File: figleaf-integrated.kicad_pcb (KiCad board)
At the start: 2 copper layers, 145 x 106 mm, 70 parts, among them J2 HRO_TYPE-C-31-M-14, J3 Battery, J9 TC2030_SWD, Q2 2N7002, SW1 PWR, SW2 RST, U1 SRV05-4, U10 MAX17048, U3 BQ24075, U8 nRF52840_moko_mk08

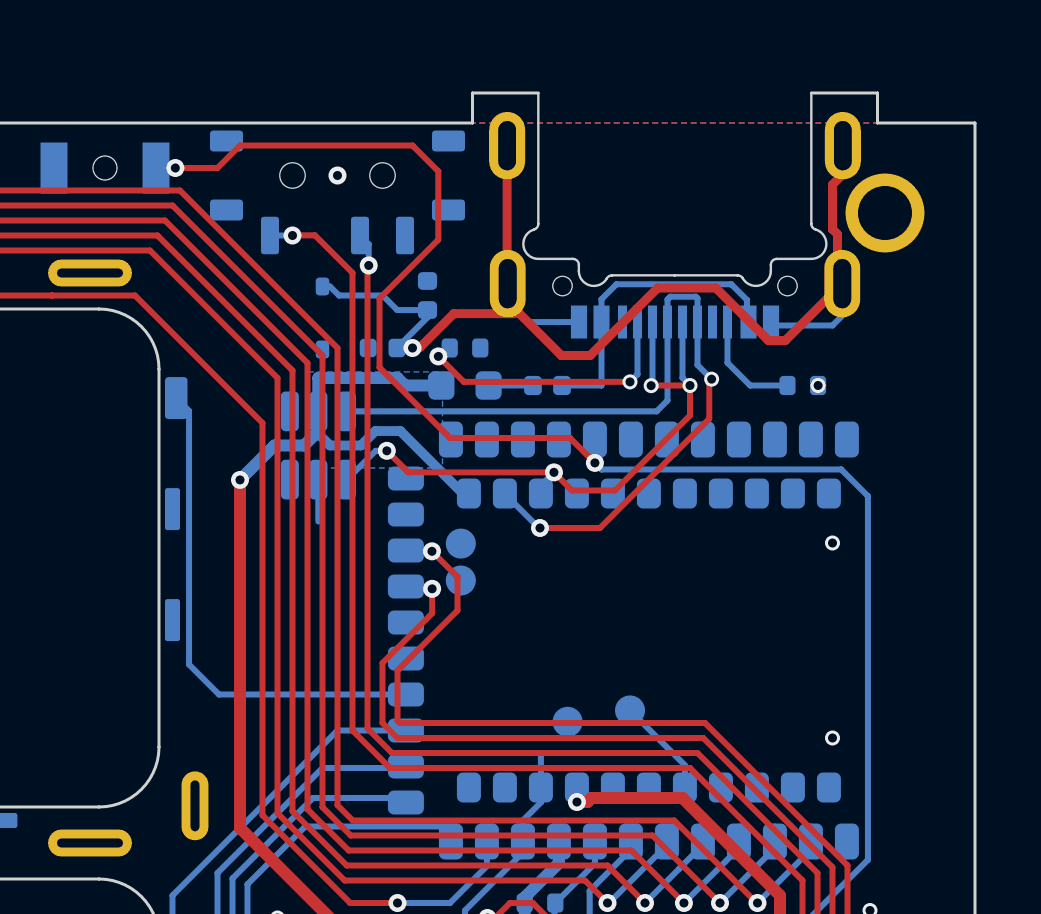
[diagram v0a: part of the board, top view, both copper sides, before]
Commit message: progress
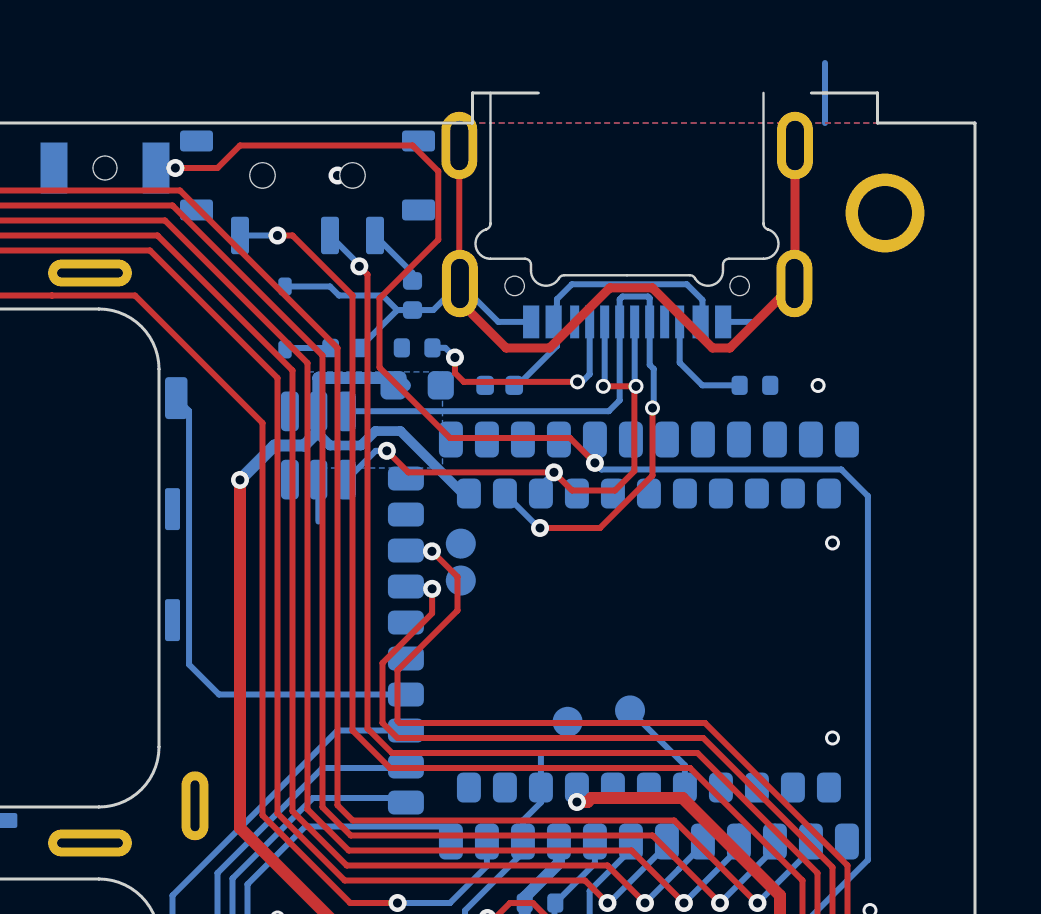
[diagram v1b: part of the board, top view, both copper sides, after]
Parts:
- moved F1 1.60 mm to (138.9, 21.2)
- moved J2 1.60 mm to (145.9, 17.9)
- moved L1 1.60 mm to (141.7, 21.2)
- moved R1 1.60 mm to (150.2, 21.2)
- moved R2 1.60 mm to (138.9, 20.0), turned to 0 degrees
- moved C1 1.25 mm to (136.5, 20.0)
- moved D1 1.25 mm to (134.5, 19.0)
- moved SW1 1.00 mm to (135.2, 14.2)
- moved L2 0.50 mm to (138.8, 18.2)
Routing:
- net GND_L: track 31.3 -> 34.9 mm
- net Earth: track 41.4 -> 38.3 mm, vias 1 -> 0
- net USB-D+: track 28.4 -> 25.9 mm
- net Net-(J2-CC1): track 9.33 -> 7.71 mm
- net +5V: track 48.7 -> 47.1 mm
- net USB-D-: track 21.0 -> 19.9 mm
- net Net-(F1-Pad1): track 1.48 -> 0.47 mm
- net VBUS: track 10.1 -> 9.30 mm
- net Net-(SW1-A): track 55.6 -> 56.2 mm
